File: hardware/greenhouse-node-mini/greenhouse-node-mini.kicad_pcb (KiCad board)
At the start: 4 copper layers, 70 x 50 mm, 43 parts, among them J1 Molex_KK_396_1x2, J2 JST_XH_2.54mm_1x2, J4 Molex_KK_396_1x2, J5 JST_XH_2.54mm_1x4, J6 PinHeader_1x04_P2.54mm, J7 PinHeader_1x04_P2.54mm, Q1 A42, SW1 SW_Push, U1 ATtiny84A-P, U2 L7805, U3 PCF8574, U4 L298HN, Y1 8MHz

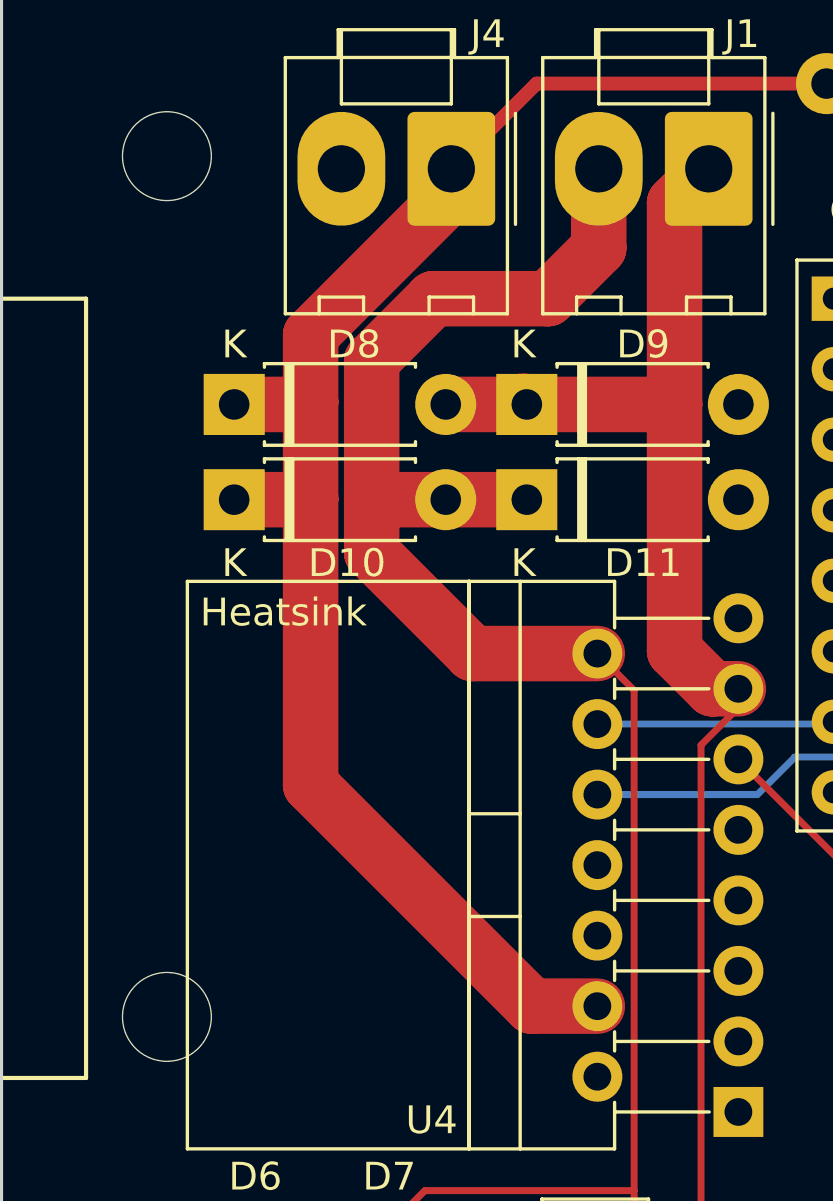
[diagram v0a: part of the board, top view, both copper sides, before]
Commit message: More track tweaking
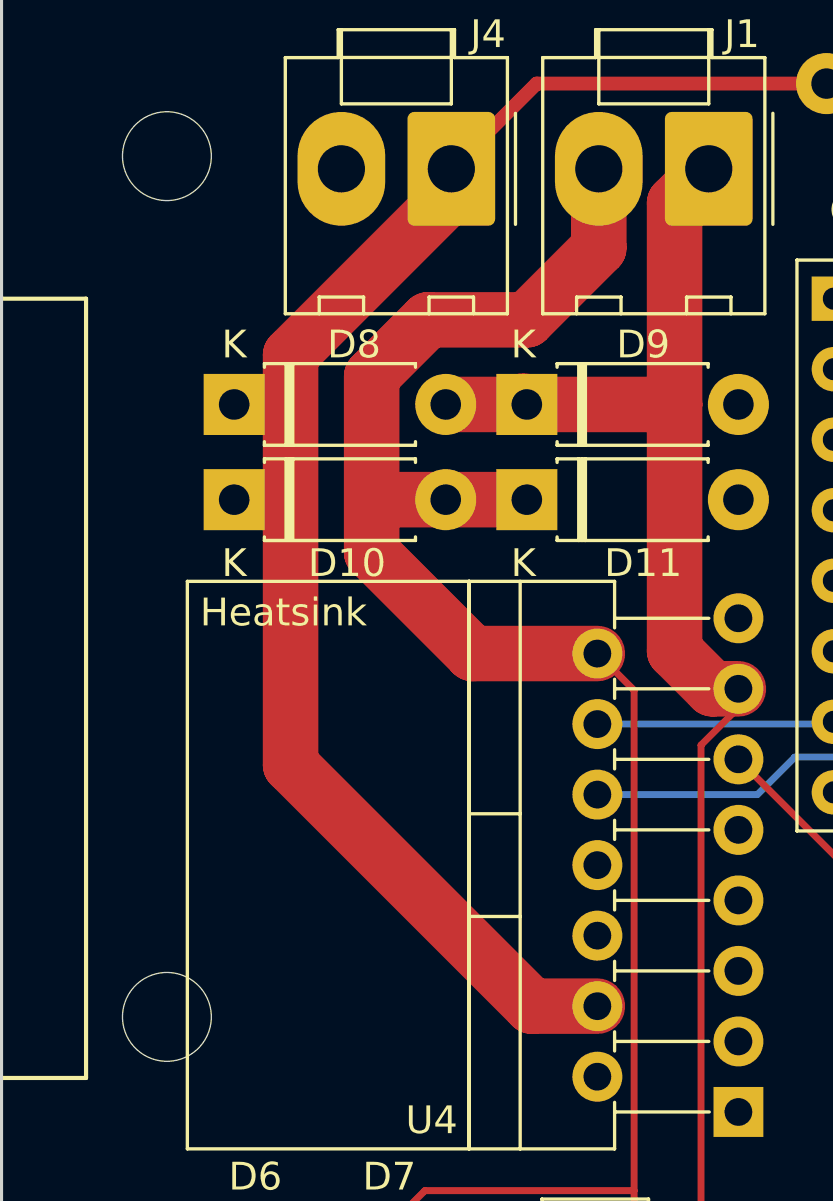
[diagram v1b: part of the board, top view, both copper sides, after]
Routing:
- net +10V: track 57.3 -> 52.4 mm
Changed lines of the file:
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@@
   (segment (start 123.317 59.309) (end 124.714 60.706) (width 0.25) (layer "F.Cu") (net 4))
   (segment (start 121.285 56.901) (end 121.285 58.6105) (width 0.25) (layer "F.Cu") (net 4))
-  (segment (start 77.17548 51.85652) (end 77.17548 55.33148) (width 2) (layer "F.Cu") (net 5))
-  (segment (start 77.13496 55.372) (end 77.17548 55.33148) (width 2) (layer "F.Cu") (net 5))
-  (segment (start 77.17548 49.444429) (end 77.17548 51.85652) (width 2) (layer "F.Cu") (net 5))
-  (segment (start 77.17548 65.64388) (end 85.1458 73.6142) (width 2) (layer "F.Cu") (net 5))
-  (segment (start 74.422 51.943) (end 77.089 51.943) (width 2) (layer "F.Cu") (net 5))
+  (segment (start 82.244 44.375909) (end 76.454 50.165909) (width 2) (layer "F.Cu") (net 5))
   (segment (start 85.1458 73.6142) (end 87.503 73.6142) (width 2) (layer "F.Cu") (net 5))
   (segment (start 95.758 40.386) (end 85.314 40.386) (width 0.5) (layer "F.Cu") (net 5))
-  (segment (start 77.089 51.943) (end 77.17548 51.85652) (width 2) (layer "F.Cu") (net 5))
+  (segment (start 76.454 64.9224) (end 85.1458 73.6142) (width 2) (layer "F.Cu") (net 5))
+  (segment (start 76.454 50.165909) (end 76.454 64.9224) (width 2) (layer "F.Cu") (net 5))
   (segment (start 85.314 40.386) (end 82.244 43.456) (width 0.5) (layer "F.Cu") (net 5))
-  (segment (start 77.17548 55.33148) (end 77.17548 65.64388) (width 2) (layer "F.Cu") (net 5))
-  (segment (start 82.244 44.375909) (end 77.17548 49.444429) (width 2) (layer "F.Cu") (net 5))
-  (segment (start 74.422 55.372) (end 77.13496 55.372) (width 2) (layer "F.Cu") (net 5))
   (segment (start 113.284 72.263) (end 112.259489 71.238489) (width 0.25) (layer "F.Cu") (net 6))
   (segment (start 112.259489 71.238489) (end 110.573633 71.238489) (width 0.25) (layer "F.Cu") (net 6))
@@
   (segment (start 75.184 81.539) (end 73.959489 82.763511) (width 0.25) (layer "F.Cu") (net 19))
   (segment (start 91.6482 62.1842) (end 90.283489 60.819489) (width 2) (layer "F.Cu") (net 19))
+  (segment (start 79.375 50.927) (end 79.375 55.372) (width 2) (layer "F.Cu") (net 20))
   (segment (start 83.0122 60.9142) (end 87.503 60.9142) (width 2) (layer "F.Cu") (net 20))
+  (segment (start 87.555 46.303) (end 84.963 48.895) (width 2) (layer "F.Cu") (net 20))
+  (segment (start 88.82752 81.71052) (end 88.82752 62.23872) (width 0.25) (layer "F.Cu") (net 20))
+  (segment (start 80.01 81.539) (end 81.29 80.259) (width 0.25) (layer "F.Cu") (net 20))
   (segment (start 87.555 43.456) (end 87.555 46.303) (width 2) (layer "F.Cu") (net 20))
-  (segment (start 81.5975 48.133) (end 79.375 50.3555) (width 2) (layer "F.Cu") (net 20))
-  (segment (start 88.82752 81.71052) (end 88.82752 62.23872) (width 0.25) (layer "F.Cu") (net 20))
-  (segment (start 79.375 57.277) (end 83.0122 60.9142) (width 2) (layer "F.Cu") (net 20))
-  (segment (start 80.01 81.539) (end 81.29 80.259) (width 0.25) (layer "F.Cu") (net 20))
-  (segment (start 87.555 46.303) (end 85.725 48.133) (width 2) (layer "F.Cu") (net 20))
-  (segment (start 79.375 50.3555) (end 79.375 55.499) (width 2) (layer "F.Cu") (net 20))
+  (segment (start 82.042 55.372) (end 79.375 55.372) (width 2) (layer "F.Cu") (net 20))
   (segment (start 88.82752 62.23872) (end 87.503 60.9142) (width 0.25) (layer "F.Cu") (net 20))
+  (segment (start 84.963 48.895) (end 81.407 48.895) (width 2) (layer "F.Cu") (net 20))
   (segment (start 91.186 84.069) (end 88.82752 81.71052) (width 0.25) (layer "F.Cu") (net 20))
   (segment (start 84.963 55.372) (end 82.042 55.372) (width 2) (layer "F.Cu") (net 20))
-  (segment (start 85.725 48.133) (end 81.5975 48.133) (width 2) (layer "F.Cu") (net 20))
-  (segment (start 79.375 55.499) (end 79.375 57.277) (width 2) (layer "F.Cu") (net 20))
-  (segment (start 82.042 55.372) (end 79.502 55.372) (width 2) (layer "F.Cu") (net 20))
+  (segment (start 79.375 57.277) (end 83.0122 60.9142) (width 2) (layer "F.Cu") (net 20))
   (segment (start 81.29 80.259) (end 88.82752 80.259) (width 0.25) (layer "F.Cu") (net 20))
-  (segment (start 79.502 55.372) (end 79.375 55.499) (width 2) (layer "F.Cu") (net 20))
+  (segment (start 81.407 48.895) (end 79.375 50.927) (width 2) (layer "F.Cu") (net 20))
+  (segment (start 79.375 55.372) (end 79.375 57.277) (width 2) (layer "F.Cu") (net 20))
   (segment (start 121.417 54.229) (end 115.072 60.574) (width 0.25) (layer "F.Cu") (net 23))
   (segment (start 123.952 54.229) (end 121.417 54.229) (width 0.25) (layer "F.Cu") (net 23))
